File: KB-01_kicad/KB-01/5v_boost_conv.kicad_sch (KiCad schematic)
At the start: 12 parts, among them U2 TPS61022

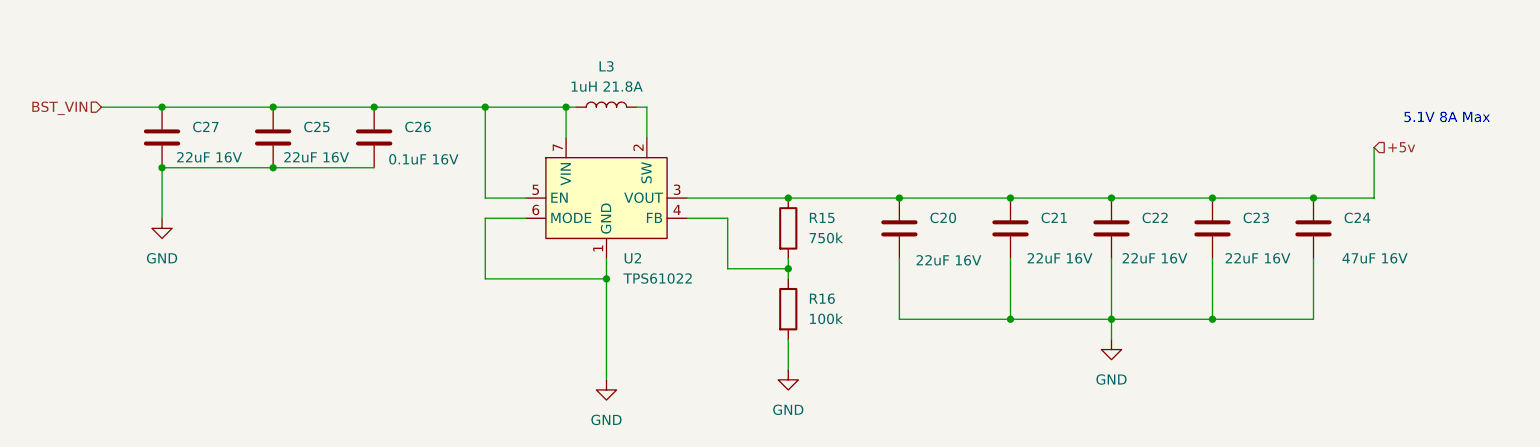
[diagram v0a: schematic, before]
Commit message: all
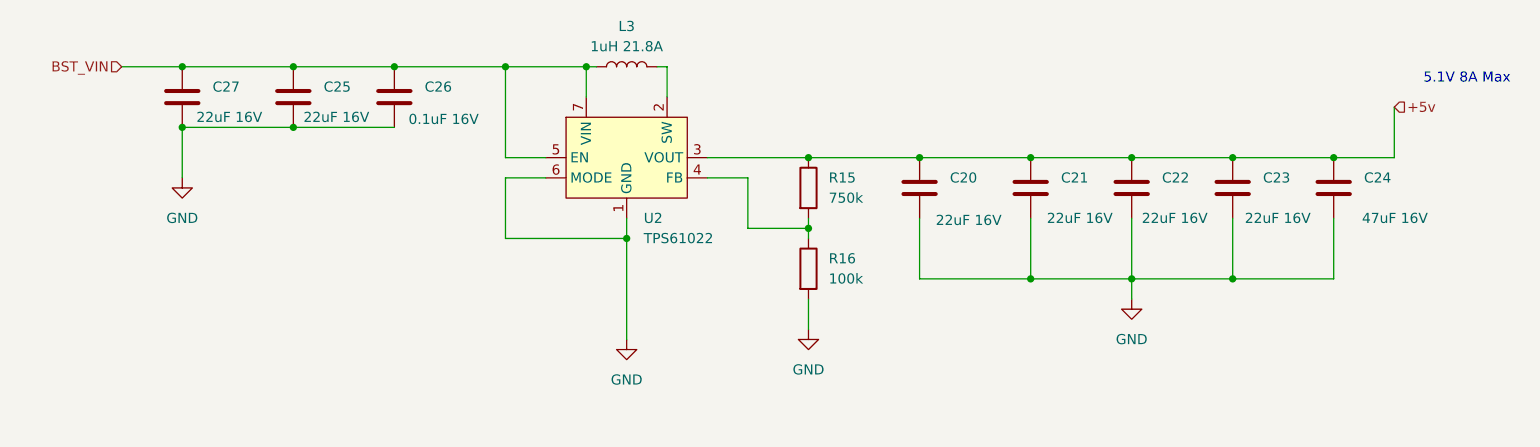
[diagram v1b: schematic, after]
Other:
- moved on the sheet: C20, C21, C22, C23, C24, C25, C26, C27, L3, R15, R16, U2

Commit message: all
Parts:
- C20, C21, C22, C23, C25, C27: mouser (none) -> 81-ZRB18AR61C226ME1L
- C26: mouser (none) -> 581-0603YC104K4T4A
- R15: mouser (none) -> 603-AC0603FR-07750KL
- R16: mouser (none) -> 603-RT0603FRE13100KL
- U2: mouser (none) -> 595-TPS61022RWUT
